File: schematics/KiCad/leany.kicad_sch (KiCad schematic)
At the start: 38 parts, among them J1 SWD, J2 SSD1306, J3 USB_C, Q1 DMG6601LVT-7, SW2 ZERO_BTN, SW3 HOLD_BTN, SW4 BOOT, U1 STM32F103C8Tx, U2 AP2112K-3.3, U3 LSM6DSO, U4 CH340C, Y1 8MHz

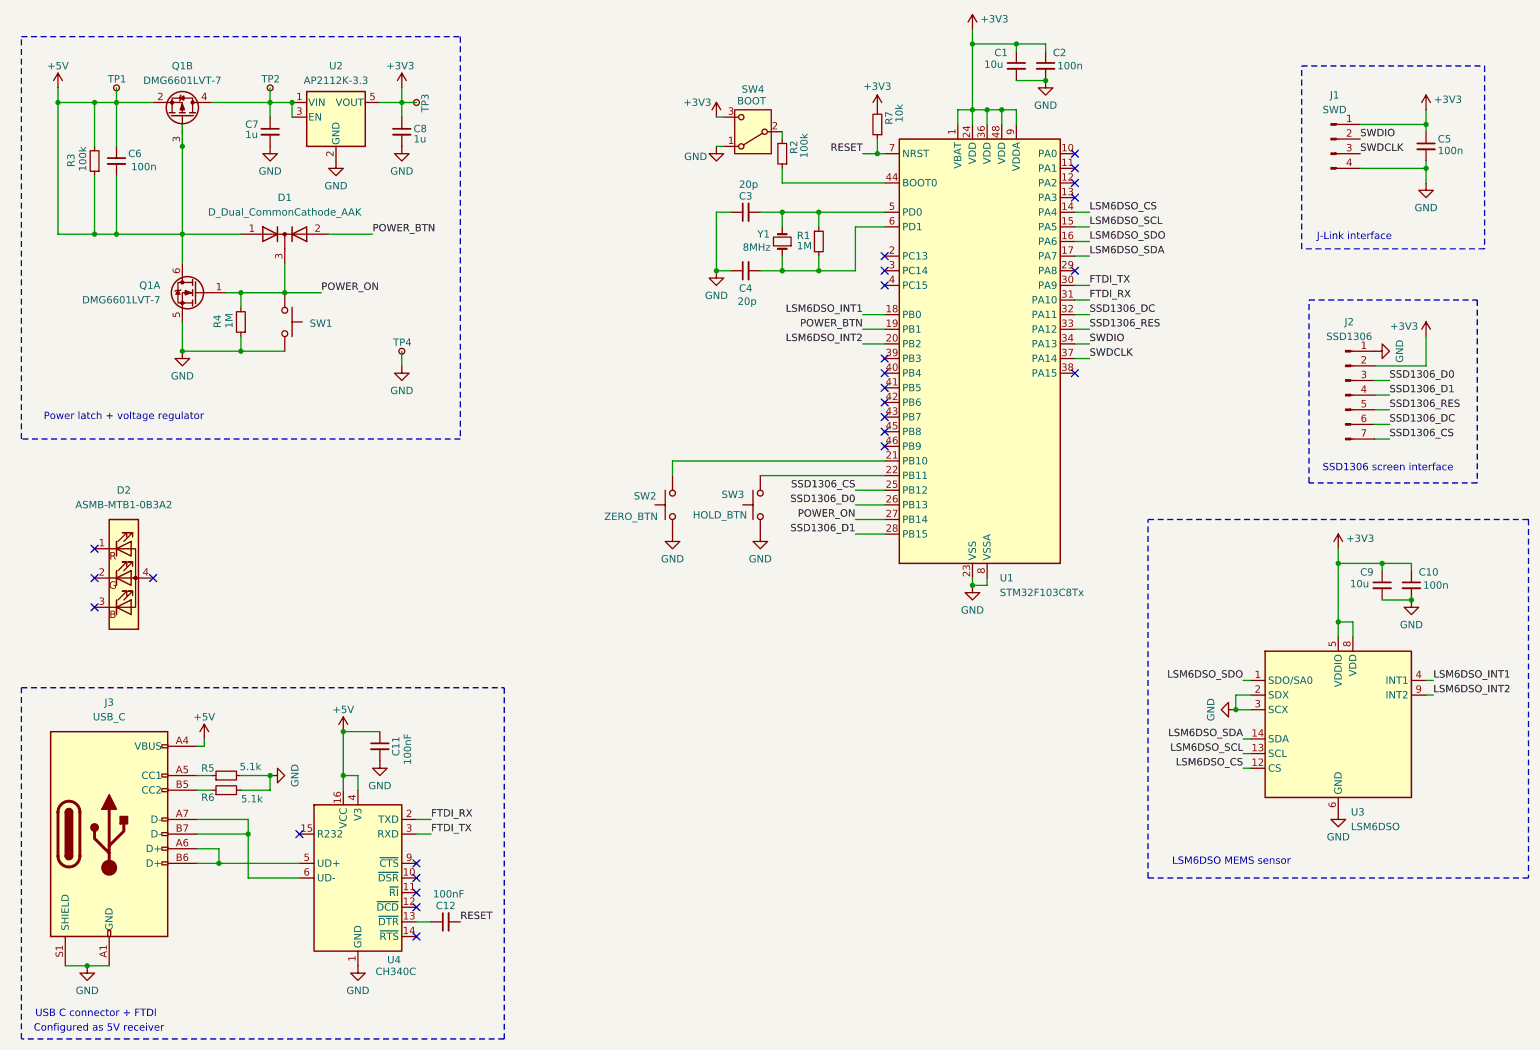
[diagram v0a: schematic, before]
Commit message: improve schematics
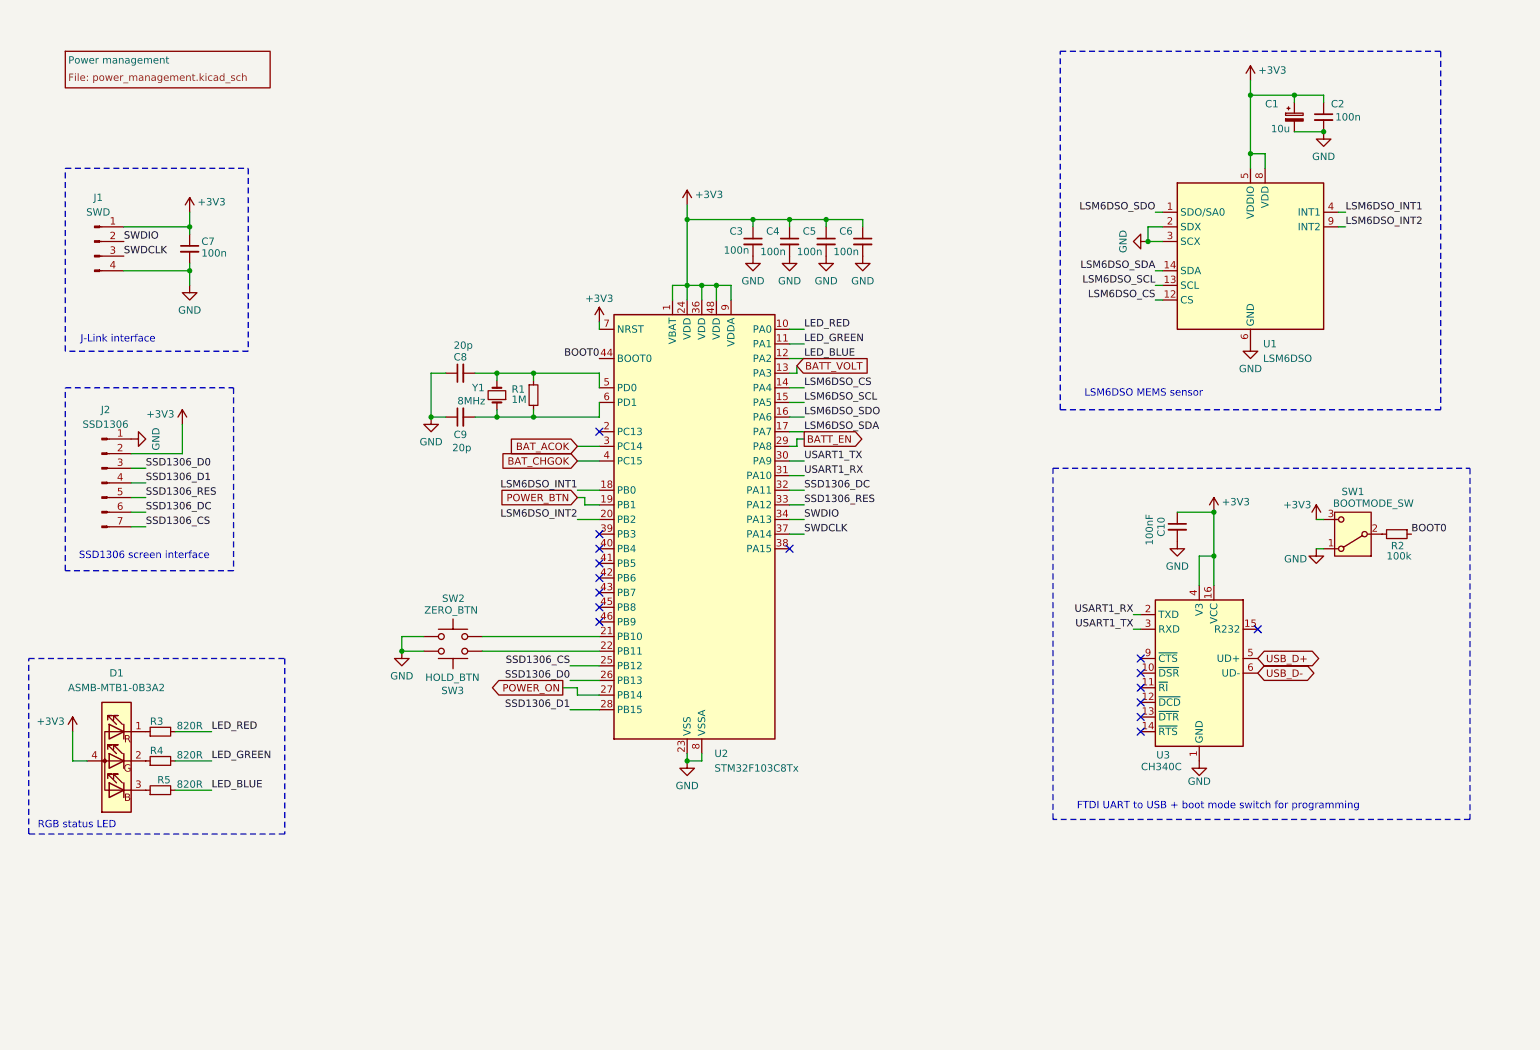
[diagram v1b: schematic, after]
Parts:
- removed C1, C9: 10u, Capacitor_SMD:C_0201_0603Metric, symbol Device:C_Small
- removed C11, C12: 100nF, Capacitor_SMD:C_0201_0603Metric, symbol Device:C_Small
- removed C2: 100n, Capacitor_SMD:C_0201_0603Metric, symbol Device:C_Small
- removed C7, C8: 1u, Capacitor_SMD:C_0201_0603Metric, symbol Device:C_Small
- removed D1: D_Dual_CommonCathode_AAK, symbol Device:D_Dual_CommonCathode_AAK
- removed J3: USB_C, Connector_USB:USB_C_Receptacle_GCT_USB4105-xx-A_16P_TopMnt_Horizontal, symbol Connector:USB_C_Receptacle_USB2.0_14P
- removed Q1: DMG6601LVT-7, Package_TO_SOT_SMD:TSOT-23-6, symbol leany-symbols:DMG6601LVT-7
- removed R6: 5.1k, Resistor_SMD:R_0603_1608Metric, symbol Device:R_Small
- removed R7: 10k, Resistor_SMD:R_0603_1608Metric, symbol Device:R_Small
- removed SW1: ~, symbol Switch:SW_Push
- removed TP1: 5V, TestPoint:TestPoint_Pad_1.0x1.0mm, symbol Connector:TestPoint_Small
- removed TP2: Vin, TestPoint:TestPoint_Pad_1.0x1.0mm, symbol Connector:TestPoint_Small
- removed TP3: 3.3V, TestPoint:TestPoint_Pad_1.0x1.0mm, symbol Connector:TestPoint_Small
- removed TP4: GND, TestPoint:TestPoint_Pad_1.0x1.0mm, symbol Connector:TestPoint_Small
- removed U2: AP2112K-3.3, Package_TO_SOT_SMD:SOT-23-5, symbol Regulator_Linear:AP2112K-3.3
- removed U4: CH340C, Package_SO:SOIC-16_3.9x9.9mm_P1.27mm, symbol Interface_USB:CH340C
- added C1: 10u, symbol Device:C_Polarized_Small
- added C10: 100nF, Capacitor_SMD:C_0201_0603Metric, symbol Device:C_Small
- added C3, C4, C5: 100n, Capacitor_SMD:C_0201_0603Metric, symbol Device:C_Small
- added U3: CH340C, Package_SO:SOIC-16_3.9x9.9mm_P1.27mm, symbol Interface_USB:CH340C
- R3: value 100k -> 820R
- R4: value 1M -> 820R
- R5: value 5.1k -> 820R
- SW1: renamed from SW4; value BOOT -> BOOTMODE_SW
- renumbered C10 to C2, C5 to C7, C3 to C8, C4 to C9, D2 to D1, U3 to U1, U1 to U2
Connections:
- net RESET is gone; now on net +3V3: U2.7 (NRST)
- net +3V3: now also C6.1, D1.4 (A), C1.1, C10.1, C3.1, C4.1, C5.1, U3.16 (VCC), U3.4 (V3)
- net GND: now also C6.2, SW3.1, C1.2, C10.2, C3.2, C4.2, C5.2, U3.1 (GND); no longer R4.1, R5.2, SW3.2
- net POWER_ON: no longer R4.2
- net at D1.1 (RK): now also R3.1
- net at D1.2 (GK): now also R4.1
- net at D1.3 (BK): now also R5.1
- net LED_RED: now reaches U2.10 (PA0)
- net LED_RED: now also R3.2
- net LED_GREEN: now reaches U2.11 (PA1)
- net LED_GREEN: now also R4.2
- net LED_BLUE: now reaches U2.12 (PA2)
- net LED_BLUE: now also R5.2
- net BATT_VOLT: now reaches U2.13 (PA3)
- net at U2.22 (PB11): now also SW3.2; no longer SW3.1
- net BATT_EN: now reaches U2.29 (PA8)
- net BAT_ACOK: now reaches U2.3 (PC14)
- net BAT_CHGOK: now reaches U2.4 (PC15)
- net BOOT0: now reaches R2.1, U2.44 (BOOT0)
- removed net +5V: C6.1, C6.2, R3.1, R3.2
- net FTDI_RX renamed USART1_RX
- net USART1_RX: now also U3.2 (TXD)
- net FTDI_TX renamed USART1_TX
- net USART1_TX: now also U3.3 (RXD)
- new net USB_D+: U3.5 (UD+)
- new net USB_D-: U3.6 (UD-)
- no-connect marks 26 -> 16
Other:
- added sheet Power management (power_management.kicad_sch)
- note added: "FTDI UART to USB + boot mode switch for programming"
- note added: "RGB status LED"
- note removed: "Configured as 5V receiver"
- note removed: "Power latch + voltage regulator"
- note removed: "USB C connector + FTDI"
- moved on the sheet: C2, C7, C8, C9, D1, J1, J2, R1, R2, SW1, SW2, SW3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
